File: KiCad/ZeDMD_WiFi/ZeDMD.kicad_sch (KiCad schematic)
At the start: 5 parts, among them J6 Conn_02x08_Odd_Even, SW6 Menu Left, SW7 Boot/Value+, SW8 Value-, SW9 Menu Right

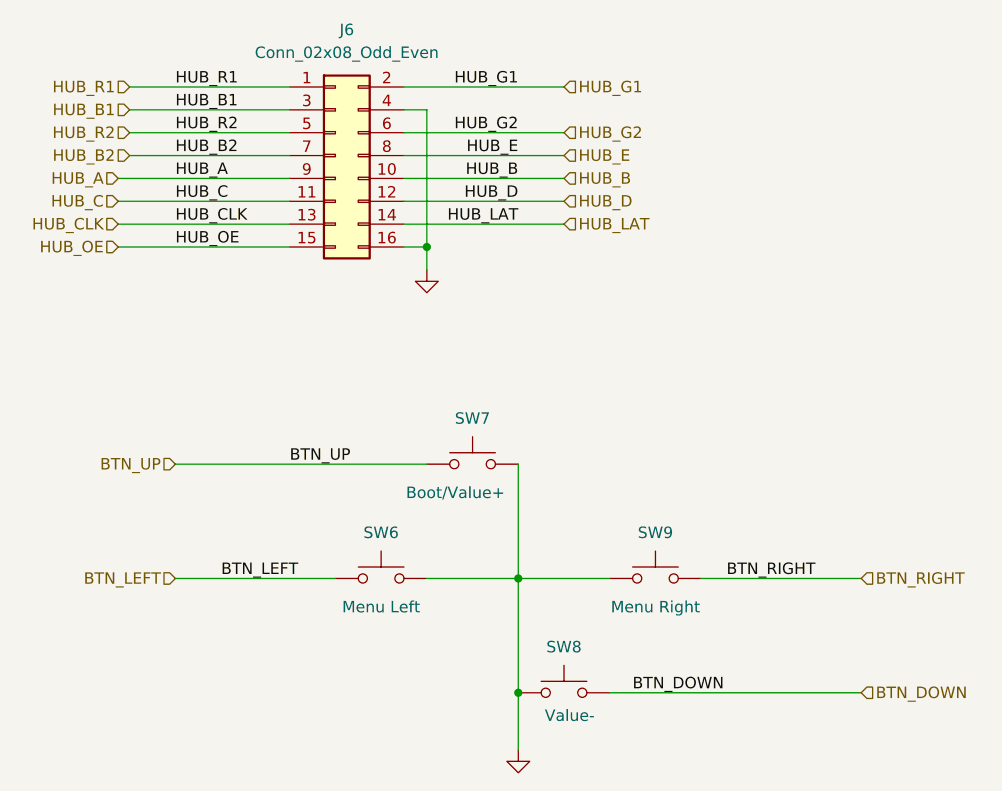
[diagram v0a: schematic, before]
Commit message: SchematicsV1.1
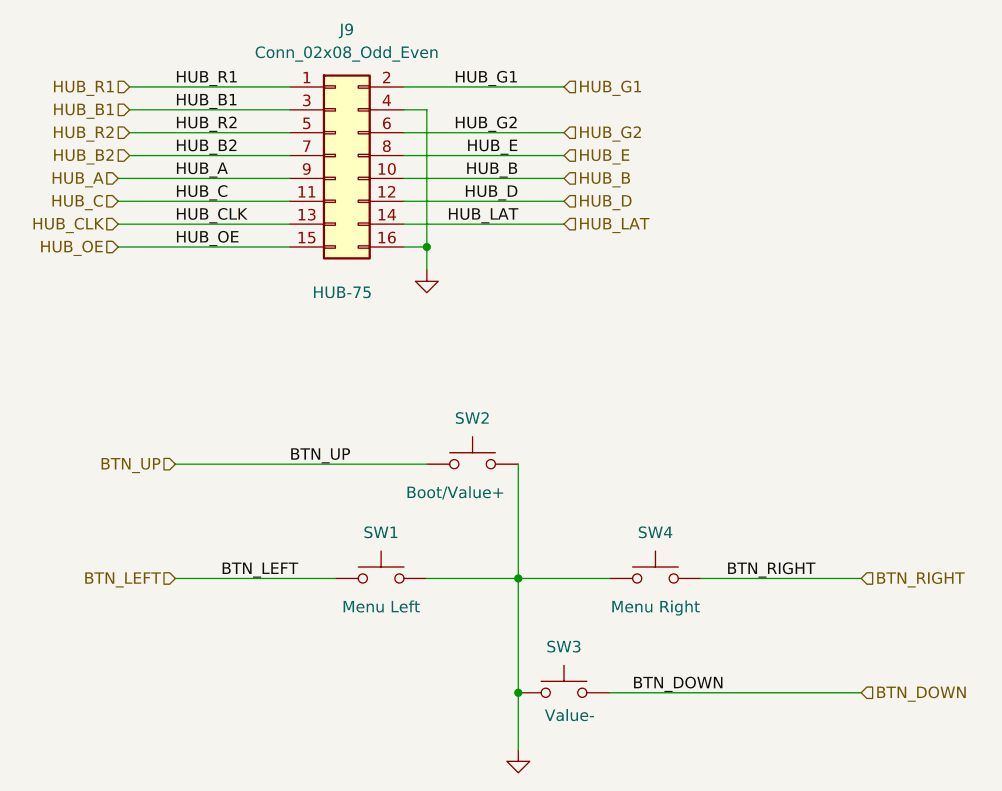
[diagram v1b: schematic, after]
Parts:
- J9: renamed from J6; footprint Connector_IDC:IDC-Header_2x08_P2.54mm_Vertical_SMD -> Connector_IDC:IDC-Header_2x08_P2.54mm_Vertical; Function (none) -> HUB-75; LCSC C601969 -> (none)
- SW1: renamed from SW6; footprint Button_Switch_SMD:SW_SPST_SKQG_WithStem -> Button_Switch_THT:SW_PUSH_6mm; LCSC C318884 -> (none)
- SW2: renamed from SW7; footprint Button_Switch_SMD:SW_SPST_SKQG_WithStem -> Button_Switch_THT:SW_PUSH_6mm; LCSC C318884 -> (none)
- SW3: renamed from SW8; footprint Button_Switch_SMD:SW_SPST_SKQG_WithStem -> Button_Switch_THT:SW_PUSH_6mm; LCSC C318884 -> (none)
- SW4: renamed from SW9; footprint Button_Switch_SMD:SW_SPST_SKQG_WithStem -> Button_Switch_THT:SW_PUSH_6mm; LCSC C318884 -> (none)
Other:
- company: (none) -> elabree
- title: (none) -> HUB75
